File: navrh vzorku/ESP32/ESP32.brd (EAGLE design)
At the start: 168.9 x 105.1 mm, 20 parts, among them U1 ESP-WROOM-32

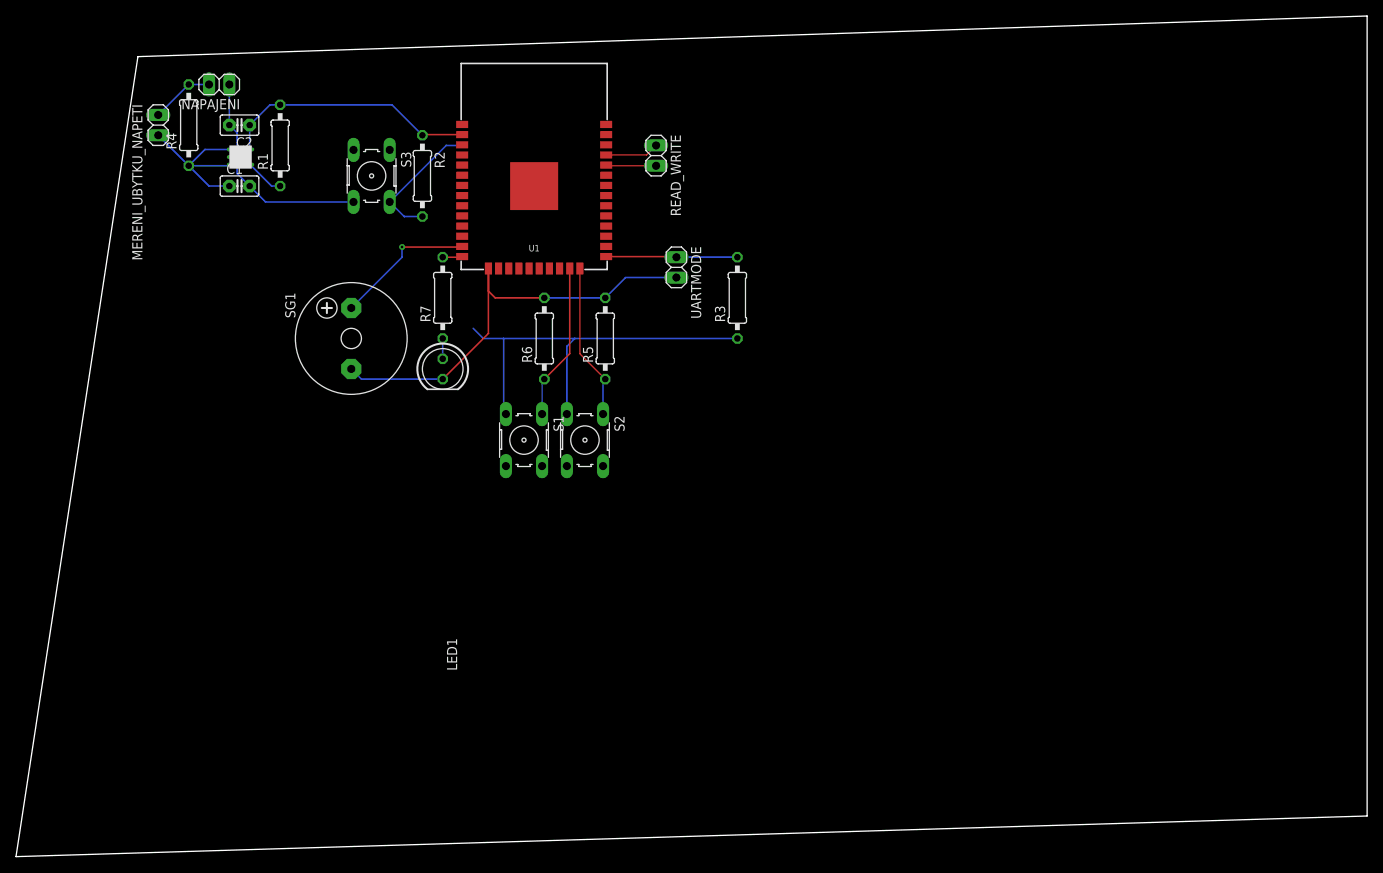
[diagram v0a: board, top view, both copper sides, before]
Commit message: funkcni vzorek ESP8266
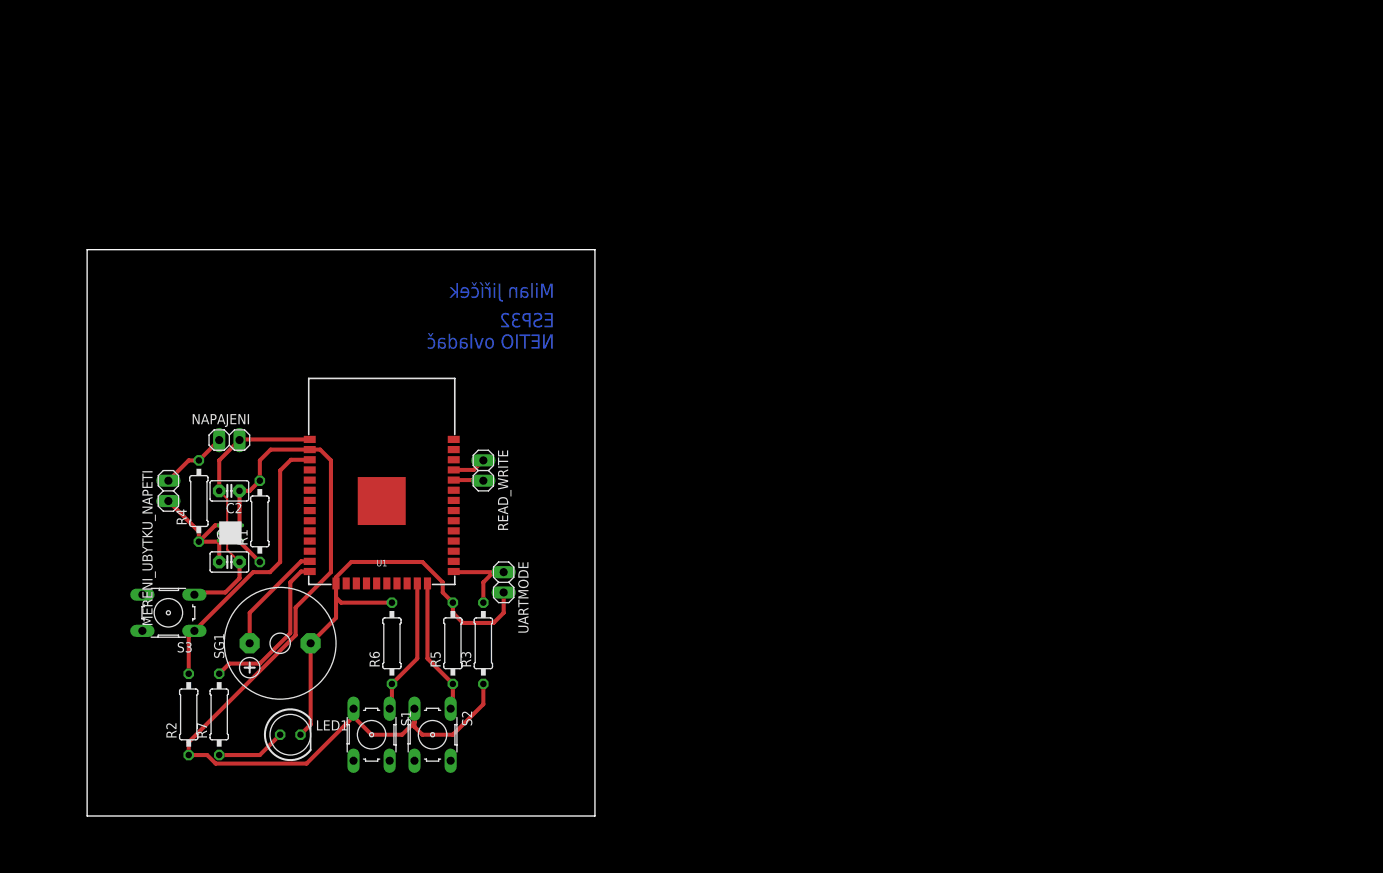
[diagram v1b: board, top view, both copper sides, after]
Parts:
- moved R2 73.4 mm to (12.7, 12.7), turned to 90 degrees
- moved S3 60.2 mm to (10.2, 25.4), turned to 180 degrees
- moved R7 59.1 mm to (16.5, 12.7)
- moved R3 53.6 mm to (49.5, 21.6)
- moved LED1 49.5 mm to (25.4, 10.2), turned to 0 degrees
- moved R1 47.1 mm to (21.6, 36.8)
- moved R4 47.0 mm to (14.0, 39.4)
- moved C1 47.0 mm to (17.8, 31.8)
- moved U$1 47.0 mm to (16.5, 36.8)
- moved C2 45.7 mm to (17.8, 40.6)
- moved MERENI_UBYTKU_NAPETI 45.7 mm to (10.2, 40.6)
- moved READ_WRITE 44.9 mm to (49.5, 43.2)
- moved UARTMODE 44.9 mm to (52.1, 29.2)
- moved NAPAJENI 44.5 mm to (17.8, 47.0)
- moved U1 43.7 mm to (36.8, 39.4)
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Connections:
- net N$3: now also S3.3; no longer S3.4
- net N$5: now also S3.1; no longer S3.2
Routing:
- net N$2: track 85.3 -> 114.9 mm
- net N$5: track 16.9 -> 35.6 mm
- net N$9: track 2.46 -> 20.3 mm
- net N$1: track 23.0 -> 15.8 mm
- net N$3: track 28.7 -> 35.6 mm
- net N$14: track 2.54 -> 8.67 mm
- net N$8: track 16.4 -> 10.6 mm
- net N$13: track 17.8 -> 14.0 mm, vias 1 -> 0
- net N$7: track 6.73 -> 4.19 mm
- net N$6: track 6.27 -> 3.73 mm
- net N$12: track 19.6 -> 17.1 mm
- net N$11: track 19.6 -> 17.1 mm
- net N$16: track 55.9 -> 58.2 mm
- net N$4: track 5.06 -> 3.71 mm
- net N$10: track 7.93 -> 8.45 mm
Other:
- board size 168.9 x 105.1 mm -> 63.5 x 70.8 mm
- board text added: "ESP32 NETIO ovladač"
- board text added: "Milan Jiříček"
